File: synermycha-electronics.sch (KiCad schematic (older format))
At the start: 0 parts

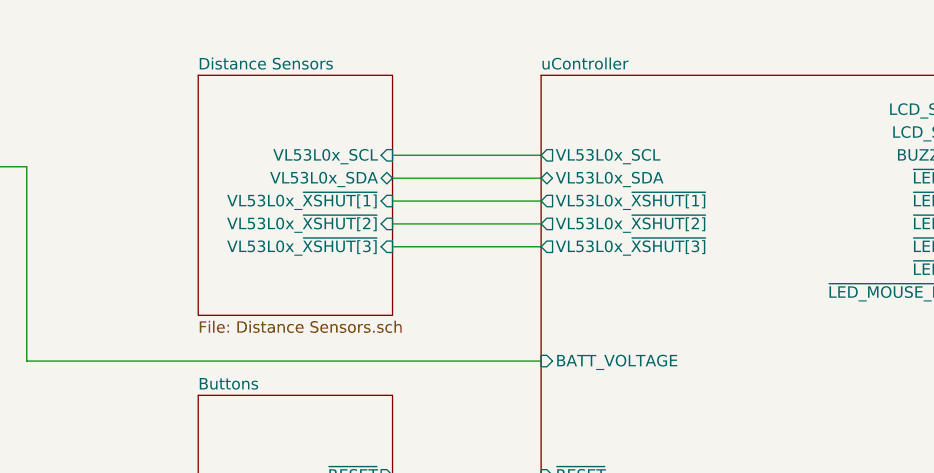
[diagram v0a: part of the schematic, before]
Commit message: Major upgrade
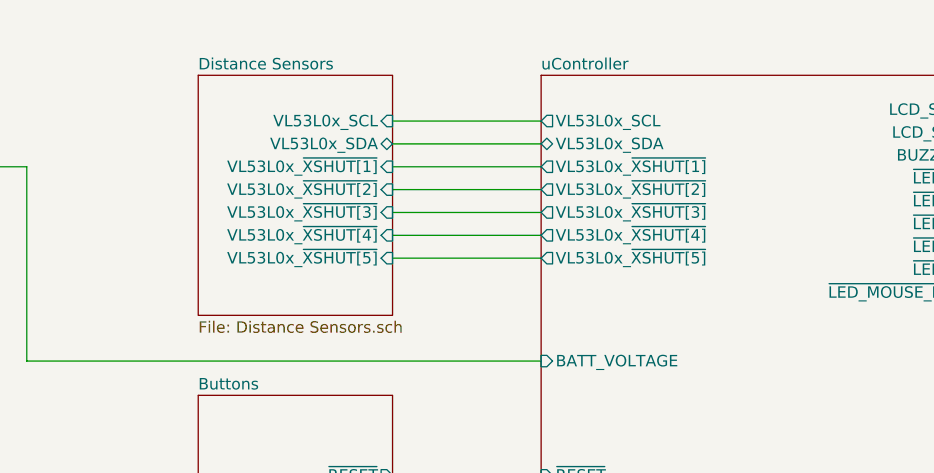
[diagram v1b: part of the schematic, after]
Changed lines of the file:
@@
 F0 "Distance Sensors" 50
 F1 "Distance Sensors.sch" 50
-F2 "VL53L0x_SCL" I R 4050 1300 50
-F3 "VL53L0x_SDA" B R 4050 1400 50
-F4 "VL53L0x_~XSHUT[1]" I R 4050 1500 50
-F5 "VL53L0x_~XSHUT[2]" I R 4050 1600 50
-F6 "VL53L0x_~XSHUT[3]" I R 4050 1700 50
+F2 "VL53L0x_SCL" I R 4050 1150 50
+F3 "VL53L0x_SDA" B R 4050 1250 50
+F4 "VL53L0x_~XSHUT[1]" I R 4050 1350 50
+F5 "VL53L0x_~XSHUT[2]" I R 4050 1450 50
+F6 "VL53L0x_~XSHUT[3]" I R 4050 1550 50
+F7 "VL53L0x_~XSHUT[4]" I R 4050 1650 50
+F8 "VL53L0x_~XSHUT[5]" I R 4050 1750 50
 $EndSheet
 $Sheet
@@
 	7350 5800 6600 5800
 Wire Wire Line
-	4050 1300 4700 1300
+	4050 1150 4700 1150
 Wire Wire Line
-	4700 1400 4050 1400
+	4700 1250 4050 1250
 Wire Wire Line
-	4050 1500 4700 1500
+	4050 1350 4700 1350
 Wire Wire Line
-	4700 1600 4050 1600
+	4700 1450 4050 1450
 Wire Wire Line
-	4050 1700 4700 1700
+	4050 1550 4700 1550
 Wire Wire Line
 	1550 1350 2450 1350
@@
 F4 "~BUTTON_DOWN" I L 4700 2900 50
 F5 "~BUTTON_OK" I L 4700 3000 50
-F6 "VL53L0x_SCL" O L 4700 1300 50
-F7 "VL53L0x_SDA" B L 4700 1400 50
-F8 "VL53L0x_~XSHUT[1]" O L 4700 1500 50
-F9 "VL53L0x_~XSHUT[2]" O L 4700 1600 50
-F10 "VL53L0x_~XSHUT[3]" O L 4700 1700 50
+F6 "VL53L0x_SCL" O L 4700 1150 50
+F7 "VL53L0x_SDA" B L 4700 1250 50
+F8 "VL53L0x_~XSHUT[1]" O L 4700 1350 50
+F9 "VL53L0x_~XSHUT[2]" O L 4700 1450 50
+F10 "VL53L0x_~XSHUT[3]" O L 4700 1550 50
 F11 "ENC_L_A" I L 4700 5600 50
 F12 "ENC_L_B" I L 4700 5700 50
@@
 F32 "DRV8835_PWM_A" O R 6600 3400 50
 F33 "DRV8835_PWM_B" O R 6600 3600 50
+F34 "VL53L0x_~XSHUT[4]" O L 4700 1650 50
+F35 "VL53L0x_~XSHUT[5]" O L 4700 1750 50
 $EndSheet
 Wire Wire Line
@@
 F10 "~LED_MOUSE_EYE" I L 7350 1900 50
 $EndSheet
+Wire Wire Line
+	4050 1650 4700 1650
+Wire Wire Line
+	4700 1750 4050 1750
 $EndSCHEMATC
